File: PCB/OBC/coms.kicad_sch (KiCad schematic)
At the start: 25 parts, among them U2 STM32F405RGTx

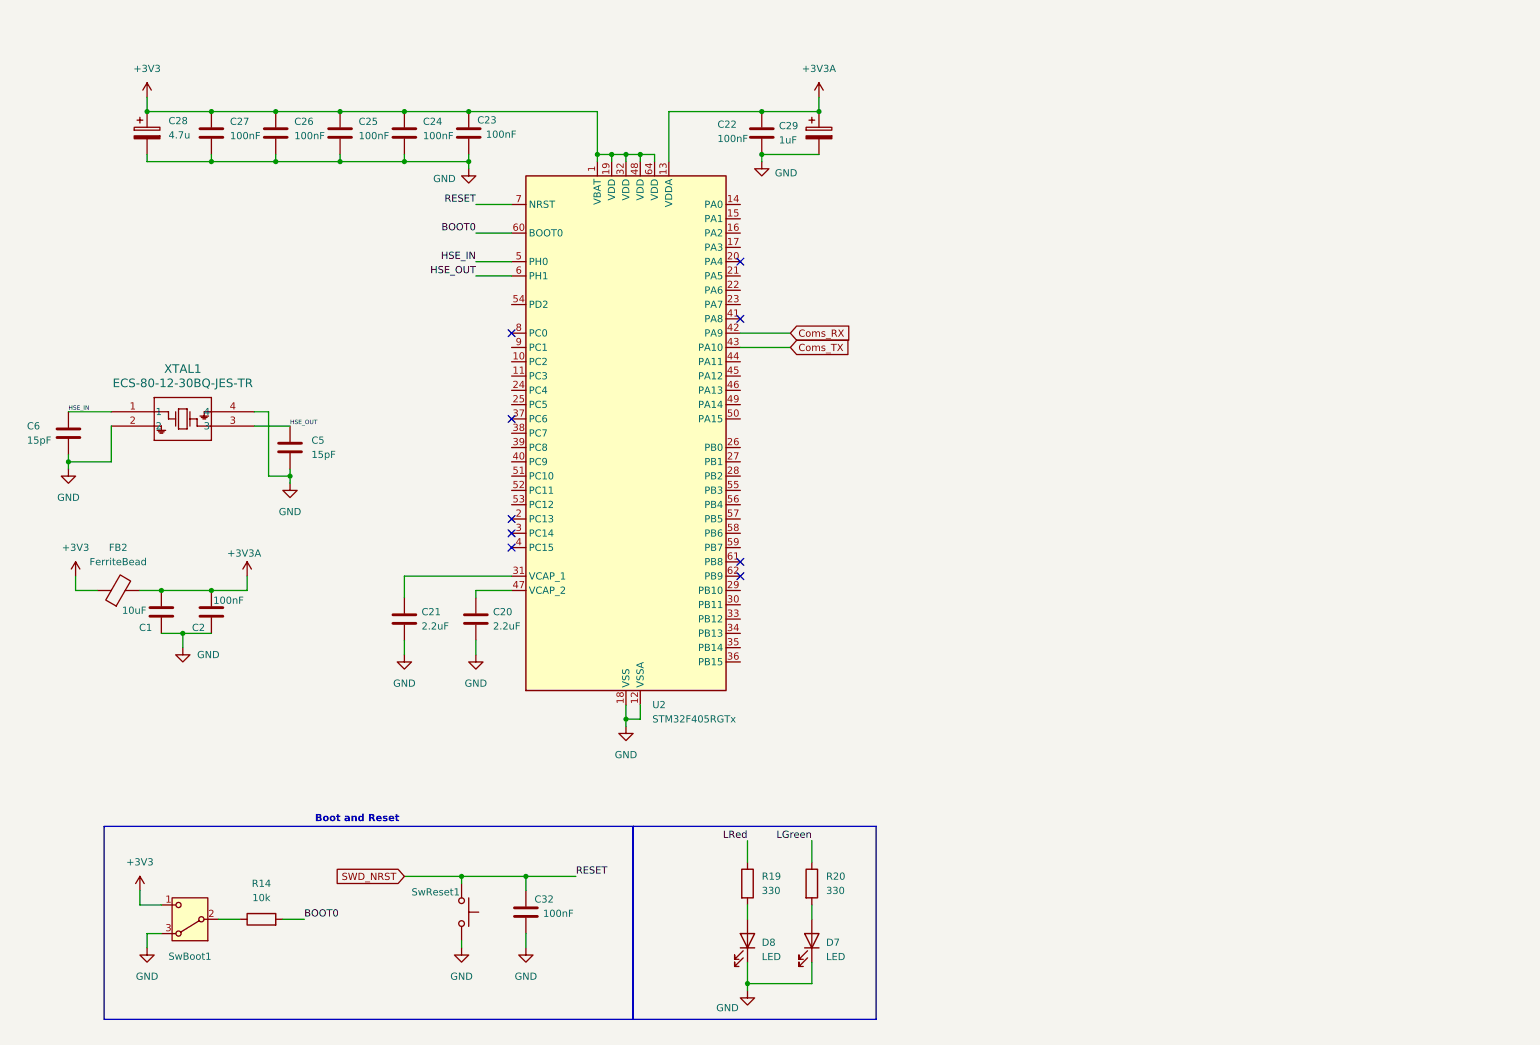
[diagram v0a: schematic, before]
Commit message: Watchdog
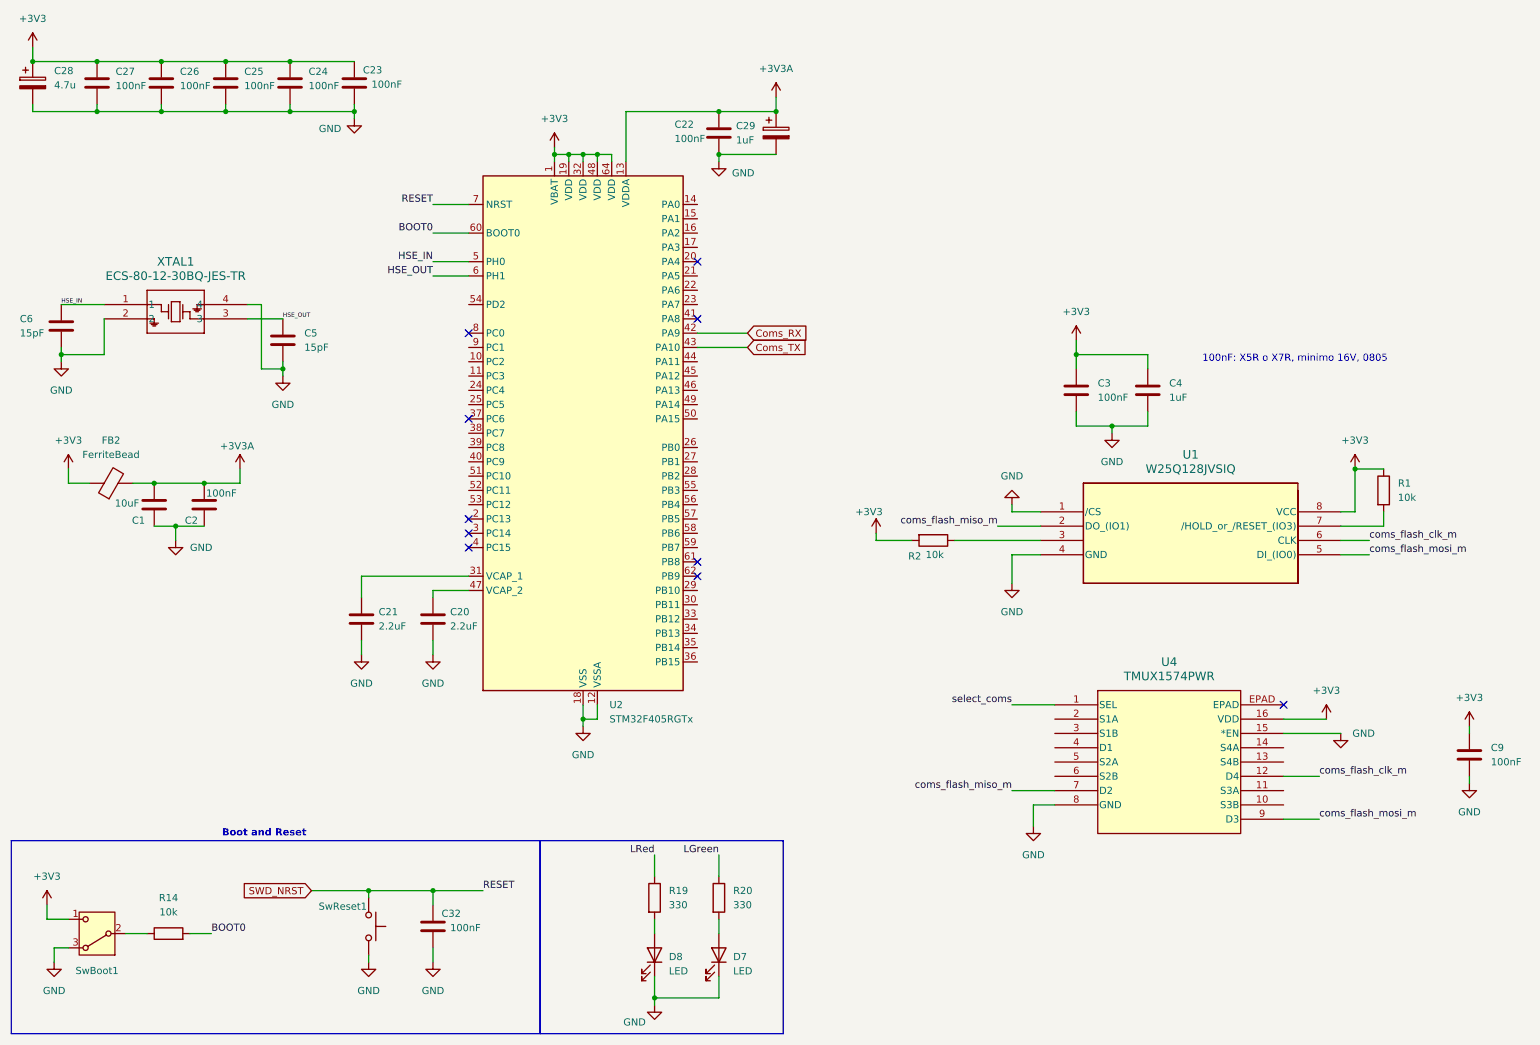
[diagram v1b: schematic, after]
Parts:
- added C3, C9: 100nF, symbol Device:C
- added C4: 1uF, symbol Device:C
- added R1, R2: 10k, symbol Device:R
- added U1: W25Q128JVSIQ, SOIC_128JVSIQ_WIN, symbol W25Q128JVSIQ:W25Q128JVSIQ
- added U4: TMUX1574PWR, PWP16_2P31X2P46_TEX, symbol TMUX1574PWR:TMUX1574PWR
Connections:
- net +3V3: now also C3.1, C4.1, C9.1, R1.1, R2.2, U1.8 (VCC), U4.16 (VDD)
- net GND: now also C3.2, C4.2, C9.2, U1.1 (/CS), U1.4 (GND), U4.15 (*EN), U4.8 (GND)
- new net: R1.2, U1.7 (/HOLD_or_/RESET_(IO3))
- new net: R2.1, U1.3
- new net coms_flash_clk_m: U1.6 (CLK), U4.12 (D4)
- new net coms_flash_miso_m: U1.2 (DO_(IO1)), U4.7 (D2)
- new net coms_flash_mosi_m: U1.5 (DI_(IO0)), U4.9 (D3)
- new net select_coms: U4.1 (SEL)
- no-connect marks 9 -> 10
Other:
- note added: "100nF: X5R o X7R, minimo 16V, 0805"
- moved on the sheet: C1, C2, C20, C21, C22, C23, C24, C25, C26, C27, C28, C29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
